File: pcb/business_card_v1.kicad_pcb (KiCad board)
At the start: 16 copper layers, 89 x 51 mm, 70 parts, among them J1 Conn_01x05_Male, J2 Conn_01x01_Male, SW1 SW_SPST, U1 MIC5504-3.3YM5, U2 STM32G030F6P6

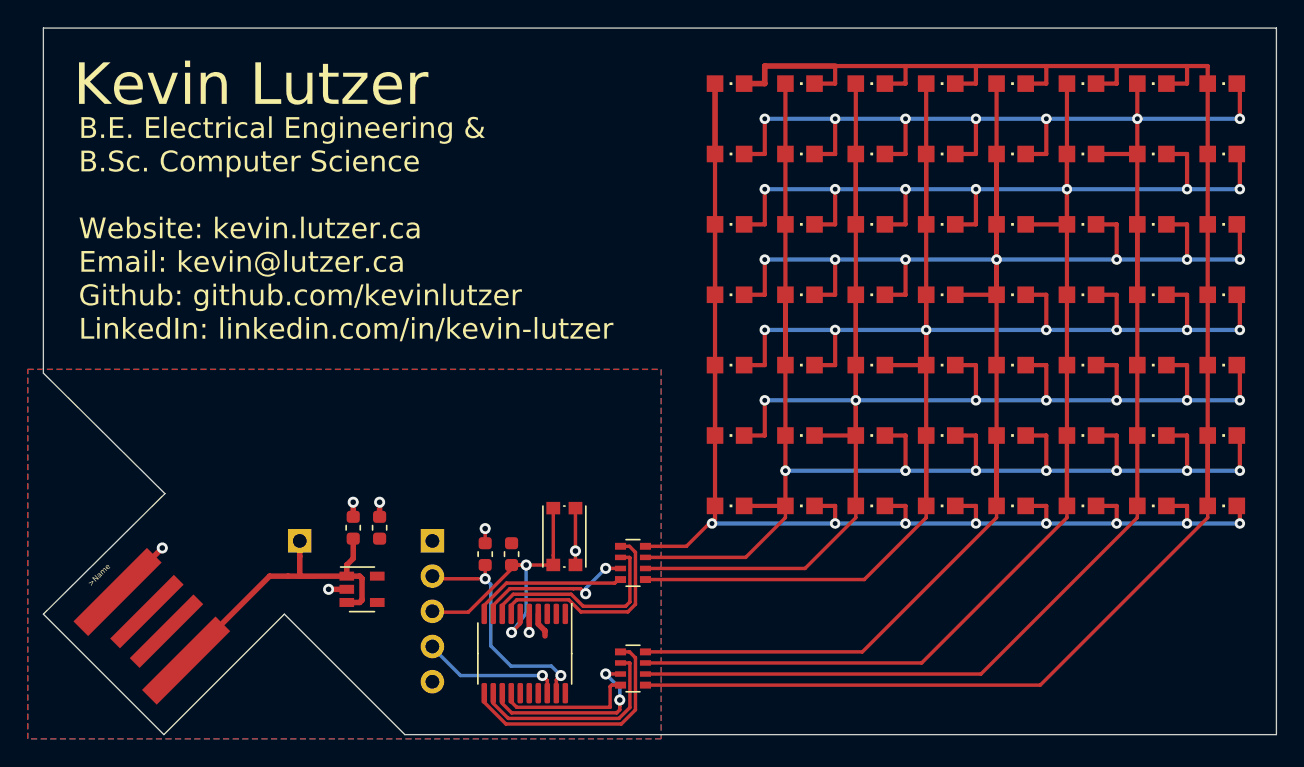
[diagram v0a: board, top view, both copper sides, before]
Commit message: update card to v4
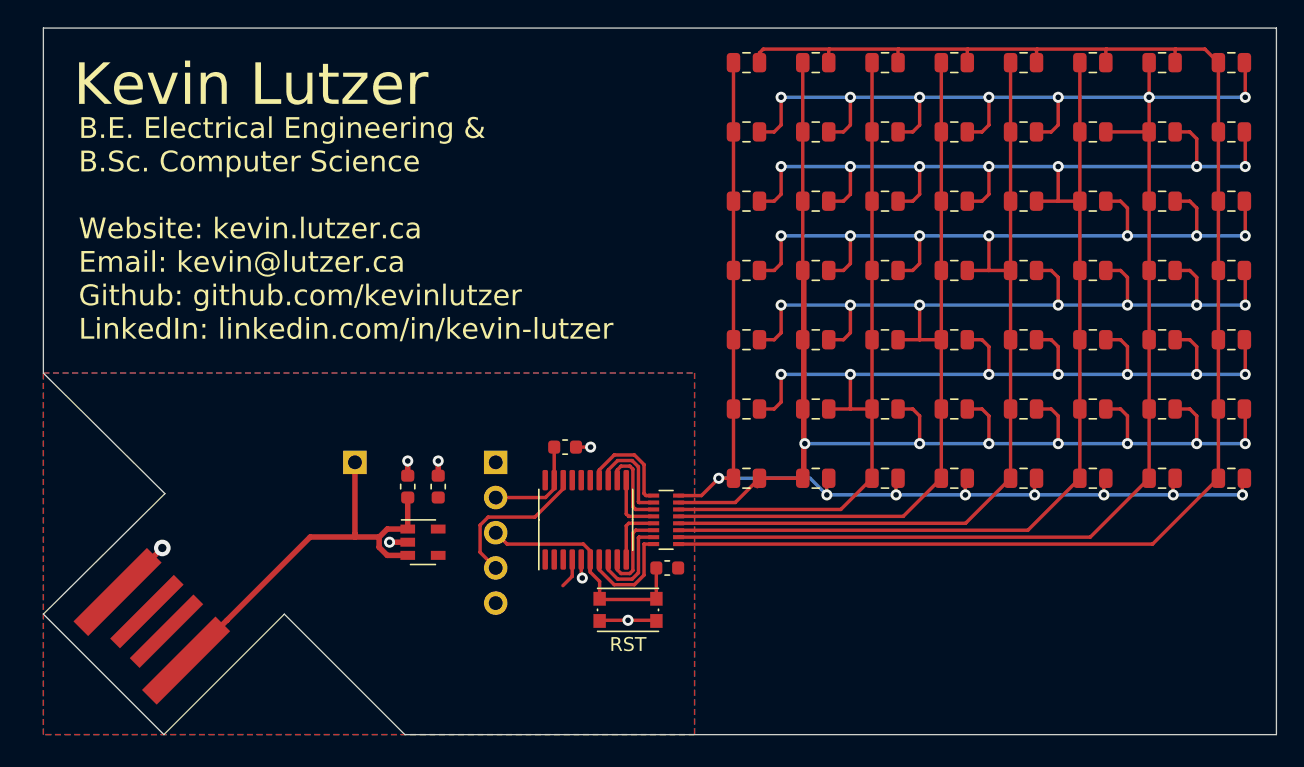
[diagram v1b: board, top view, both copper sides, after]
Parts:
- removed LED1, LED10, LED11, LED12, LED13, LED14, LED15, LED16, LED17, LED18, LED19, LED2, LED20, LED21, LED22, LED23, LED24, LED25, LED26, LED27, LED28, LED29, LED3, LED30, LED31, LED32, LED33, LED34, LED35, LED36, LED37, LED38, LED39, LED4, LED40, LED41, LED42, LED43, LED44, LED45, LED46, LED47, LED48, LED49, LED5, LED50, LED51, LED52, LED53, LED54, LED55, LED56, LED6, LED7, LED8, LED9: LEDCHIPLED_0805, business_card_v1:CHIPLED_0805
- removed R10: 10K, Resistor_SMD:R_0603_1608Metric
- removed RN2: R_Pack04, Resistor_SMD:R_Array_Convex_4x0603
- added D1: LED, Resistor_SMD:R_0805_2012Metric, F.Cu at (154.8, 82.0)
- added D10: LED, Resistor_SMD:R_0805_2012Metric, F.Cu at (159.8, 87.0)
- added D11: LED, Resistor_SMD:R_0805_2012Metric, F.Cu at (164.8, 87.0)
- added D12: LED, Resistor_SMD:R_0805_2012Metric, F.Cu at (169.8, 87.0)
- added D13: LED, Resistor_SMD:R_0805_2012Metric, F.Cu at (174.8, 87.0)
- added D14: LED, Resistor_SMD:R_0805_2012Metric, F.Cu at (179.8, 87.0)
- added D15: LED, Resistor_SMD:R_0805_2012Metric, F.Cu at (184.8, 87.0)
- added D16: LED, Resistor_SMD:R_0805_2012Metric, F.Cu at (189.8, 87.0)
- added D17: LED, Resistor_SMD:R_0805_2012Metric, F.Cu at (154.8, 92.0)
- added D18: LED, Resistor_SMD:R_0805_2012Metric, F.Cu at (159.8, 92.0)
- added D19: LED, Resistor_SMD:R_0805_2012Metric, F.Cu at (164.8, 92.0)
- added D2: LED, Resistor_SMD:R_0805_2012Metric, F.Cu at (159.8, 82.0)
- added D20: LED, Resistor_SMD:R_0805_2012Metric, F.Cu at (169.8, 92.0)
- added D21: LED, Resistor_SMD:R_0805_2012Metric, F.Cu at (174.8, 92.0)
- added D22: LED, Resistor_SMD:R_0805_2012Metric, F.Cu at (179.8, 92.0)
- added D23: LED, Resistor_SMD:R_0805_2012Metric, F.Cu at (184.8, 92.0)
- added D24: LED, Resistor_SMD:R_0805_2012Metric, F.Cu at (189.8, 92.0)
- added D25: LED, Resistor_SMD:R_0805_2012Metric, F.Cu at (154.8, 97.0)
- added D26: LED, Resistor_SMD:R_0805_2012Metric, F.Cu at (159.8, 97.0)
- added D27: LED, Resistor_SMD:R_0805_2012Metric, F.Cu at (164.8, 97.0)
- added D28: LED, Resistor_SMD:R_0805_2012Metric, F.Cu at (169.8, 97.0)
- added D29: LED, Resistor_SMD:R_0805_2012Metric, F.Cu at (174.8, 97.0)
- added D3: LED, Resistor_SMD:R_0805_2012Metric, F.Cu at (164.8, 82.0)
- added D30: LED, Resistor_SMD:R_0805_2012Metric, F.Cu at (179.8, 97.0)
- added D31: LED, Resistor_SMD:R_0805_2012Metric, F.Cu at (184.8, 97.0)
- added D32: LED, Resistor_SMD:R_0805_2012Metric, F.Cu at (189.8, 97.0)
- added D33: LED, Resistor_SMD:R_0805_2012Metric, F.Cu at (154.8, 102.0)
- added D34: LED, Resistor_SMD:R_0805_2012Metric, F.Cu at (159.8, 102.0)
- added D35: LED, Resistor_SMD:R_0805_2012Metric, F.Cu at (164.8, 102.0)
- added D36: LED, Resistor_SMD:R_0805_2012Metric, F.Cu at (169.8, 102.0)
- added D37: LED, Resistor_SMD:R_0805_2012Metric, F.Cu at (174.8, 102.0)
- added D38: LED, Resistor_SMD:R_0805_2012Metric, F.Cu at (179.8, 102.0)
- added D39: LED, Resistor_SMD:R_0805_2012Metric, F.Cu at (184.8, 102.0)
- added D4: LED, Resistor_SMD:R_0805_2012Metric, F.Cu at (169.8, 82.0)
- added D40: LED, Resistor_SMD:R_0805_2012Metric, F.Cu at (189.8, 102.0)
- added D41: LED, Resistor_SMD:R_0805_2012Metric, F.Cu at (154.8, 107.0)
- added D42: LED, Resistor_SMD:R_0805_2012Metric, F.Cu at (159.8, 107.0)
- added D43: LED, Resistor_SMD:R_0805_2012Metric, F.Cu at (164.8, 107.0)
- added D44: LED, Resistor_SMD:R_0805_2012Metric, F.Cu at (169.8, 107.0)
- added D45: LED, Resistor_SMD:R_0805_2012Metric, F.Cu at (174.8, 107.0)
- added D46: LED, Resistor_SMD:R_0805_2012Metric, F.Cu at (179.8, 107.0)
- added D47: LED, Resistor_SMD:R_0805_2012Metric, F.Cu at (184.8, 107.0)
- added D48: LED, Resistor_SMD:R_0805_2012Metric, F.Cu at (189.8, 107.0)
- added D49: LED, Resistor_SMD:R_0805_2012Metric, F.Cu at (154.8, 112.0)
- added D5: LED, Resistor_SMD:R_0805_2012Metric, F.Cu at (174.8, 82.0)
- added D50: LED, Resistor_SMD:R_0805_2012Metric, F.Cu at (159.8, 112.0)
- added D51: LED, Resistor_SMD:R_0805_2012Metric, F.Cu at (164.8, 112.0)
- added D52: LED, Resistor_SMD:R_0805_2012Metric, F.Cu at (169.8, 112.0)
- added D53: LED, Resistor_SMD:R_0805_2012Metric, F.Cu at (174.8, 112.0)
- added D54: LED, Resistor_SMD:R_0805_2012Metric, F.Cu at (179.8, 112.0)
- added D55: LED, Resistor_SMD:R_0805_2012Metric, F.Cu at (184.8, 112.0)
- added D56: LED, Resistor_SMD:R_0805_2012Metric, F.Cu at (189.8, 112.0)
- added D6: LED, Resistor_SMD:R_0805_2012Metric, F.Cu at (179.8, 82.0)
- added D7: LED, Resistor_SMD:R_0805_2012Metric, F.Cu at (184.8, 82.0)
- added D8: LED, Resistor_SMD:R_0805_2012Metric, F.Cu at (189.8, 82.0)
- added D9: LED, Resistor_SMD:R_0805_2012Metric, F.Cu at (154.8, 87.0)
- added R2: 10K, Resistor_SMD:R_0603_1608Metric, F.Cu at (149.0, 118.5)
- J2: footprint Connector_PinSocket_2.54mm:PinSocket_1x01_P2.54mm_Vertical -> Connector_PinHeader_2.54mm:PinHeader_1x01_P2.54mm_Vertical
- RN1: value R_Pack04 -> R_Pack08; footprint Resistor_SMD:R_Array_Convex_4x0603 -> Resistor_SMD:R_Array_Convex_8x0602
- moved U2 10.6 mm to (143.1, 115.0), turned to 90 degrees
- moved R1 9.64 mm to (141.7, 109.8), turned to 0 degrees
- moved J1 7.28 mm to (136.7, 110.8)
- moved SW1 7.01 mm to (146.2, 121.5), turned to 0 degrees
- moved J2 6.94 mm to (126.5, 110.8), turned to 180 degrees
- moved U1 5.56 mm to (131.4, 116.6)
- moved C3 5.17 mm to (132.5, 112.6)
- moved C2 4.93 mm to (130.3, 112.6)
- moved REF** 4.23 mm to (137.0, 86.5)
- moved RN1 3.92 mm to (148.9, 115.0)
- moved REF** 0.25 mm to (114.7, 86.4)
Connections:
- RN1 pad 1: PINA -> PINH
- RN1 pad 2: PINB -> PING
- RN1 pad 3: PINC -> PINF
- RN1 pad 4: PIND -> PINE
- RN1 pad 5: Net-(LED12-PadA) -> PIND
- RN1 pad 6: Net-(LED11-PadA) -> PINC
- RN1 pad 7: Net-(LED10-PadA) -> PINB
- RN1 pad 8: Net-(LED1-PadA) -> PINA
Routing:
- net Net-(LED10-PadC): track 136.8 -> 0.00 mm, vias 7 -> 0
- net Net-(LED14-PadA): track 136.4 -> 0.00 mm, vias 7 -> 0
- net Net-(LED13-PadA): track 136.1 -> 0.00 mm, vias 7 -> 0
- net Net-(LED1-PadC): track 134.6 -> 0.00 mm
- net Net-(LED12-PadA): track 128.9 -> 0.00 mm, vias 7 -> 0
- net Net-(D10-Pad1): track 0.00 -> 125.4 mm, vias 0 -> 7
- net Net-(LED11-PadA): track 123.5 -> 0.00 mm, vias 7 -> 0
- net Net-(D14-Pad2): track 0.00 -> 122.8 mm, vias 0 -> 7
- net Net-(D13-Pad2): track 0.00 -> 117.2 mm, vias 0 -> 7
- net Net-(D12-Pad2): track 0.00 -> 112.4 mm, vias 0 -> 7
- net Net-(D1-Pad1): track 0.00 -> 111.2 mm
- net Net-(D10-Pad2): track 0.00 -> 110.7 mm, vias 0 -> 7
- net Net-(D11-Pad2): track 0.00 -> 108.0 mm, vias 0 -> 7
- net Net-(LED10-PadA): track 106.4 -> 0.00 mm, vias 7 -> 0
- net Net-(LED1-PadA): track 104.9 -> 0.00 mm, vias 8 -> 0
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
